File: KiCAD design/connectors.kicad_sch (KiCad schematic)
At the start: 8 parts, among them J201 Conn_02x19_Odd_Even, J202 Conn_01x03_Female, J203 Conn_01x03_Female, J204 Conn_02x19_Odd_Even, J205 JST BATTERY, J206 JST SENS TOF 2, J208 JST SENS TOF 1, J401 Conn_02x06_Top_Bottom

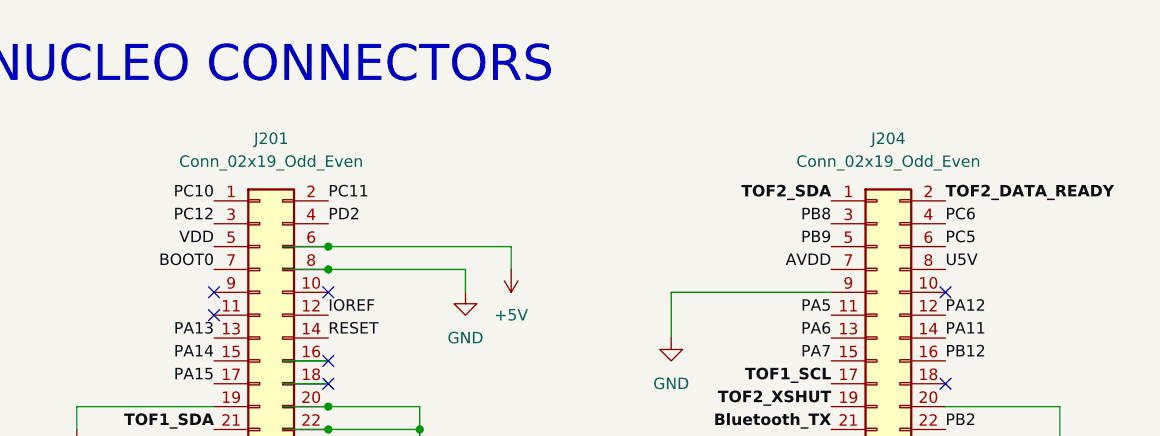
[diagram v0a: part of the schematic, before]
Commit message: Fixes
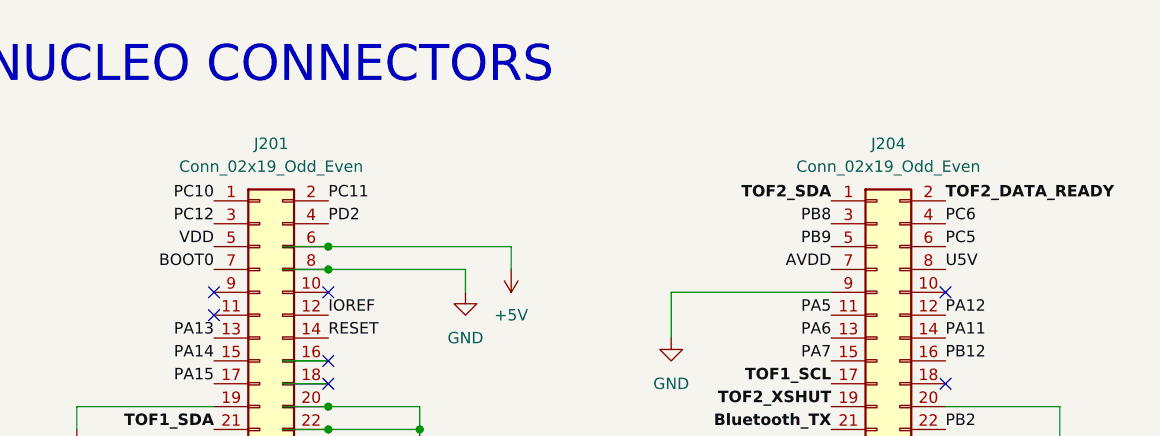
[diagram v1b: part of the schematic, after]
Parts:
- J201, J204: footprint Connector_JST:JST_PUD_B38B-PUDSS_2x19_P2.00mm_Vertical -> Connector_PinHeader_2.54mm:PinHeader_2x19_P2.54mm_Vertical
- J202, J203: footprint Connector_JST:JST_XH_B3B-XH-A_1x03_P2.50mm_Vertical -> Connector_JST:JST_EH_B3B-EH-A_1x03_P2.50mm_Vertical
- J206, J208: footprint Connector_JST:JST_XH_B6B-XH-A_1x06_P2.50mm_Vertical -> Connector_PinHeader_2.54mm:PinHeader_1x06_P2.54mm_Vertical
- J401: footprint (none) -> Connector_PinHeader_2.54mm:PinHeader_2x06_P2.54mm_Vertical
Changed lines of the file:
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@@
       (effects (font (size 1.27 1.27)) (justify left))
     )
-    (property "Footprint" "Connector_JST:JST_XH_B3B-XH-A_1x03_P2.50mm_Vertical" (id 2) (at 66.04 157.48 0)
+    (property "Footprint" "Connector_JST:JST_EH_B3B-EH-A_1x03_P2.50mm_Vertical" (id 2) (at 66.04 157.48 0)
       (effects (font (size 1.27 1.27)) hide)
     )
@@
   (symbol (lib_id "Connector_Generic:Conn_02x19_Odd_Even") (at 111.76 55.88 0) (unit 1)
     (in_bom yes) (on_board yes) (fields_autoplaced)
-    (property "Reference" "J204" (id 0) (at 113.03 26.1112 0))
-    (property "Value" "Conn_02x19_Odd_Even" (id 1) (at 113.03 28.6512 0))
-    (property "Footprint" "Connector_JST:JST_PUD_B38B-PUDSS_2x19_P2.00mm_Vertical" (id 2) (at 111.76 55.88 0)
+    (property "Reference" "J204" (id 0) (at 113.03 26.67 0))
+    (property "Value" "Conn_02x19_Odd_Even" (id 1) (at 113.03 29.21 0))
+    (property "Footprint" "Connector_PinHeader_2.54mm:PinHeader_2x19_P2.54mm_Vertical" (id 2) (at 111.76 55.88 0)
       (effects (font (size 1.27 1.27)) hide)
     )
@@
       (effects (font (size 1.27 1.27)) (justify left))
     )
-    (property "Footprint" "Connector_JST:JST_XH_B6B-XH-A_1x06_P2.50mm_Vertical" (id 2) (at 203.2 58.42 0)
+    (property "Footprint" "Connector_PinHeader_2.54mm:PinHeader_1x06_P2.54mm_Vertical" (id 2) (at 203.2 58.42 0)
       (effects (font (size 1.27 1.27)) hide)
     )
@@
   (symbol (lib_id "Connector_Generic:Conn_02x19_Odd_Even") (at 43.18 55.88 0) (unit 1)
     (in_bom yes) (on_board yes) (fields_autoplaced)
-    (property "Reference" "J201" (id 0) (at 44.45 26.1112 0))
-    (property "Value" "Conn_02x19_Odd_Even" (id 1) (at 44.45 28.6512 0))
-    (property "Footprint" "Connector_JST:JST_PUD_B38B-PUDSS_2x19_P2.00mm_Vertical" (id 2) (at 43.18 55.88 0)
+    (property "Reference" "J201" (id 0) (at 44.45 26.67 0))
+    (property "Value" "Conn_02x19_Odd_Even" (id 1) (at 44.45 29.21 0))
+    (property "Footprint" "Connector_PinHeader_2.54mm:PinHeader_2x19_P2.54mm_Vertical" (id 2) (at 43.18 55.88 0)
       (effects (font (size 1.27 1.27)) hide)
     )
@@
       (effects (font (size 1.27 1.27)) (justify left))
     )
-    (property "Footprint" "Connector_JST:JST_XH_B6B-XH-A_1x06_P2.50mm_Vertical" (id 2) (at 257.175 59.055 0)
+    (property "Footprint" "Connector_PinHeader_2.54mm:PinHeader_1x06_P2.54mm_Vertical" (id 2) (at 257.175 59.055 0)
       (effects (font (size 1.27 1.27)) hide)
     )
@@
       (effects (font (size 1.27 1.27)) (justify left))
     )
-    (property "Footprint" "Connector_JST:JST_XH_B3B-XH-A_1x03_P2.50mm_Vertical" (id 2) (at 66.04 137.16 0)
+    (property "Footprint" "Connector_JST:JST_EH_B3B-EH-A_1x03_P2.50mm_Vertical" (id 2) (at 66.04 137.16 0)
       (effects (font (size 1.27 1.27)) hide)
     )
@@
     (property "Reference" "J401" (id 0) (at 223.52 124.46 0))
     (property "Value" "Conn_02x06_Top_Bottom" (id 1) (at 223.52 127 0))
-    (property "Footprint" "" (id 2) (at 222.25 135.89 0)
-      (effects (font (size 1.27 1.27)) hide)
-    )
+    (property "Footprint" "Connector_PinHeader_2.54mm:PinHeader_2x06_P2.54mm_Vertical" (id 2) (at 222.25 135.89 0)
+      (effects (font (size 1.27 1.27)) hide)
+    )
